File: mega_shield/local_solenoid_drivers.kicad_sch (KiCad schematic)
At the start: 0 parts

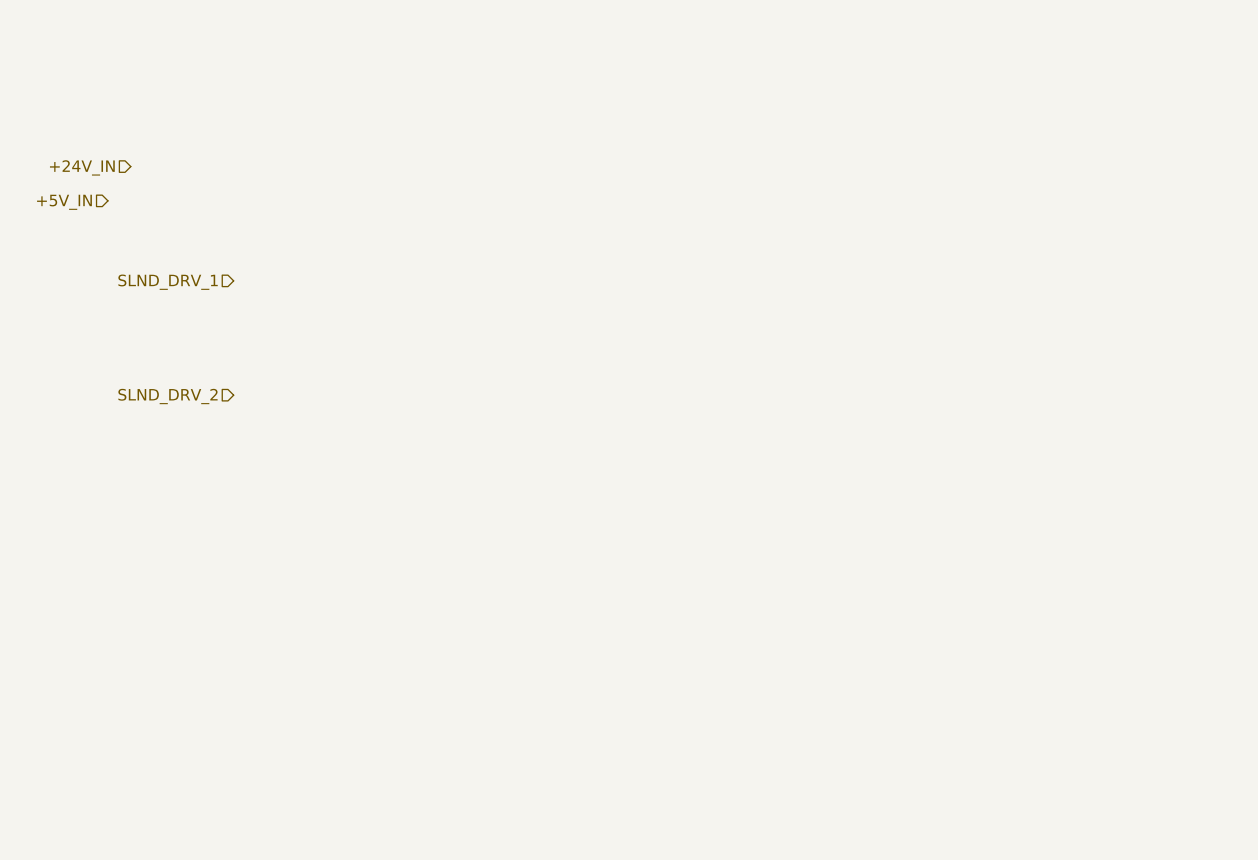
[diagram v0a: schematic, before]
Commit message: Added solenoid N-channel mosfet, led indicator, snubber diode and polyfuse.
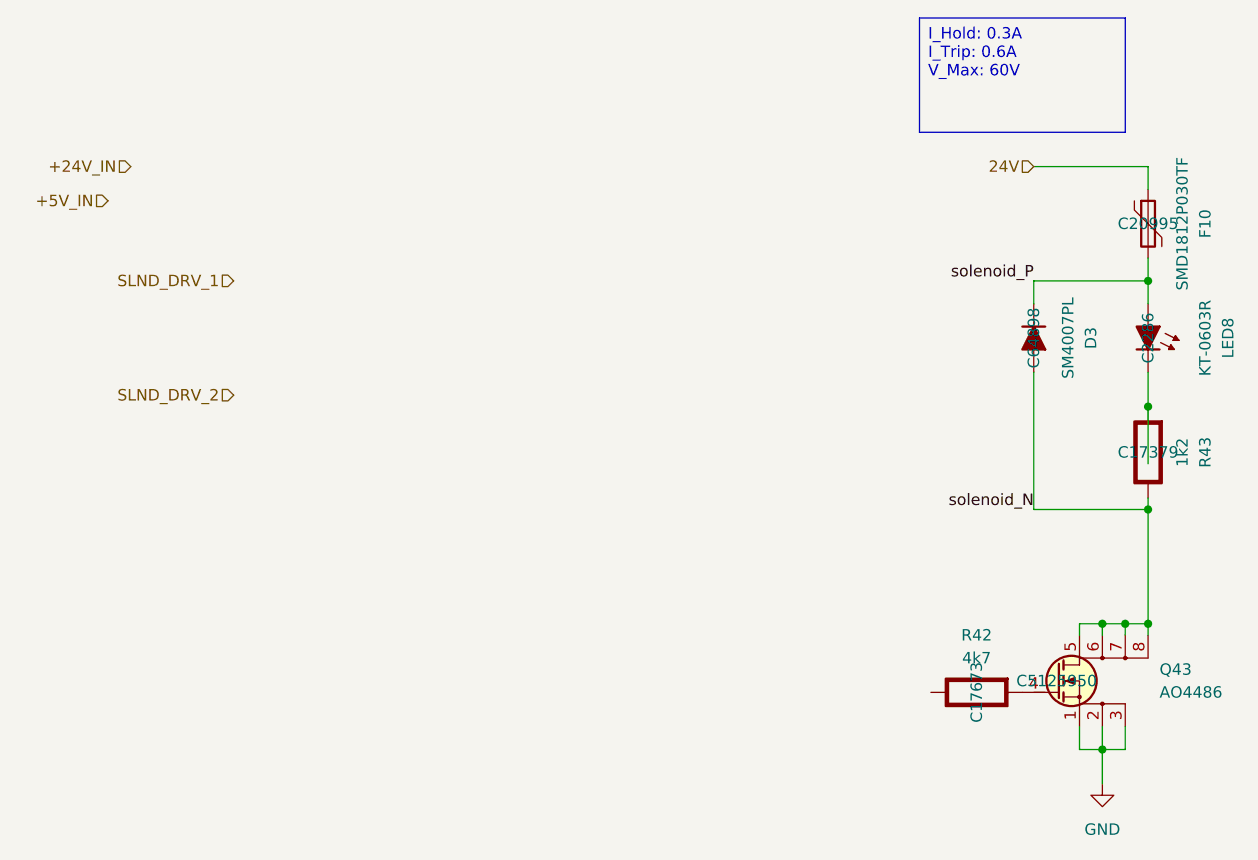
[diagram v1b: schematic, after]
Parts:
- added D3: SM4007PL, PCM_Diode_SMD_AKL:D_SOD-123F, symbol PCM_Diode_AKL:SM4007PL
- added F10: SMD1812P030TF, Fuse:Fuse_1812_4532Metric_Pad1.30x3.40mm_HandSolder, symbol Device:Polyfuse
- added LED8: KT-0603R, PCM_LED_SMD_AKL:LED_0201_0603Metric, symbol PCM_LED_AKL:LED_1.8mm_SMD
- added Q43: AO4486, PCM_Package_SO_AKL:SO-8_3.9x4.9mm_P1.27mm, symbol PCM_Transistor_MOSFET_AKL:AO4486
- added R42: 4k7, Resistor_SMD:R_0805_2012Metric_Pad1.20x1.40mm_HandSolder, symbol PCM_Elektuur:R
- added R43: 1k2, Resistor_SMD:R_0805_2012Metric_Pad1.20x1.40mm_HandSolder, symbol PCM_Elektuur:R
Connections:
- new net: Q43.4 (G), R42.2 (-)
- new net: LED8.1 (K), R43.2 (-)
- new net 24V: F10.1
- new net GND: Q43.1 (S), Q43.2 (S), Q43.3 (S)
- new net solenoid_N: D3.2 (A), Q43.5 (D), Q43.6 (D), Q43.7 (D), Q43.8 (D), R43.1 (+)
- new net solenoid_P: D3.1 (K), F10.2, LED8.2 (A)
